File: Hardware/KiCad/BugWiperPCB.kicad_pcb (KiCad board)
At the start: 2 copper layers, 121.9 x 50.8 mm, 56 parts, among them J1 UJ20-C-H-G-SMT-1-P16-TR, Q1 NMOS_SO-8, U1 ESP32-S3-WROOM-1, U2 BTN9960LV, U3 BTN9960LV, U5 WE-TVS-82400102

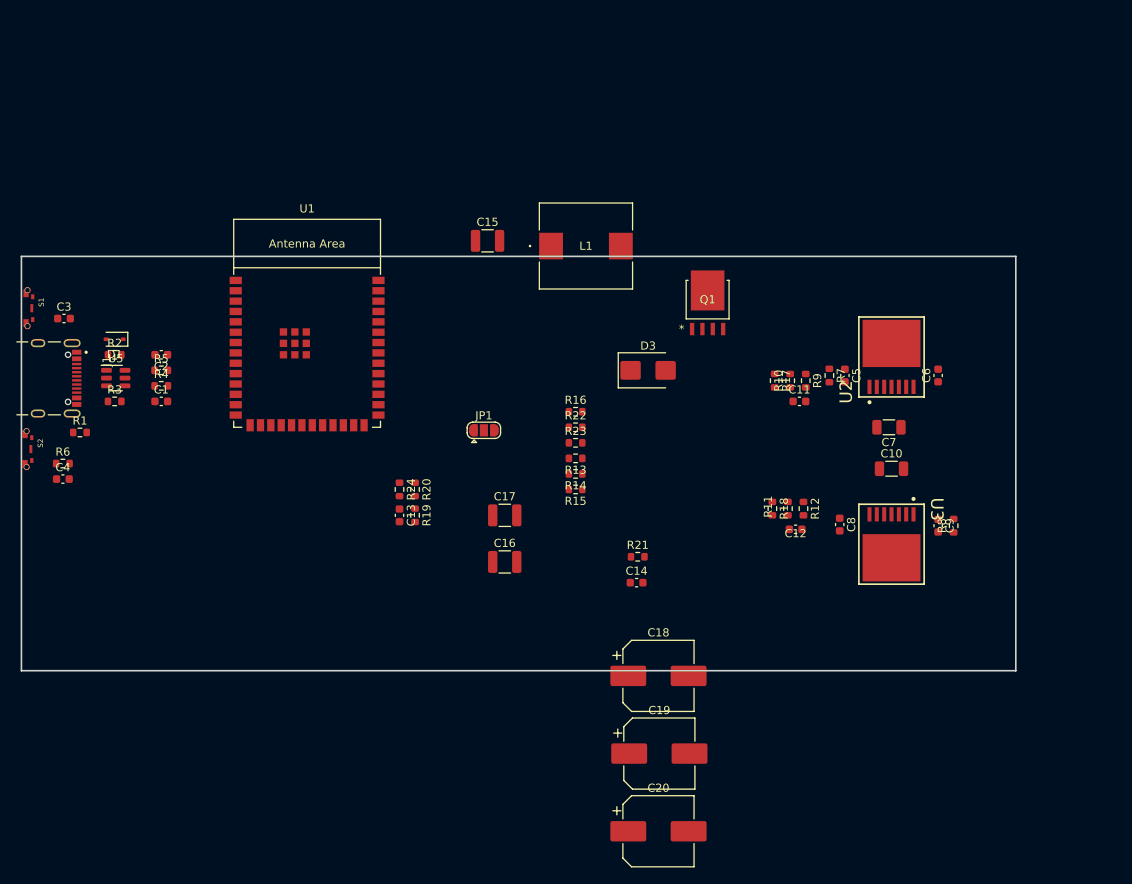
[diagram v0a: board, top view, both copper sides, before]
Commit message: Update PCB
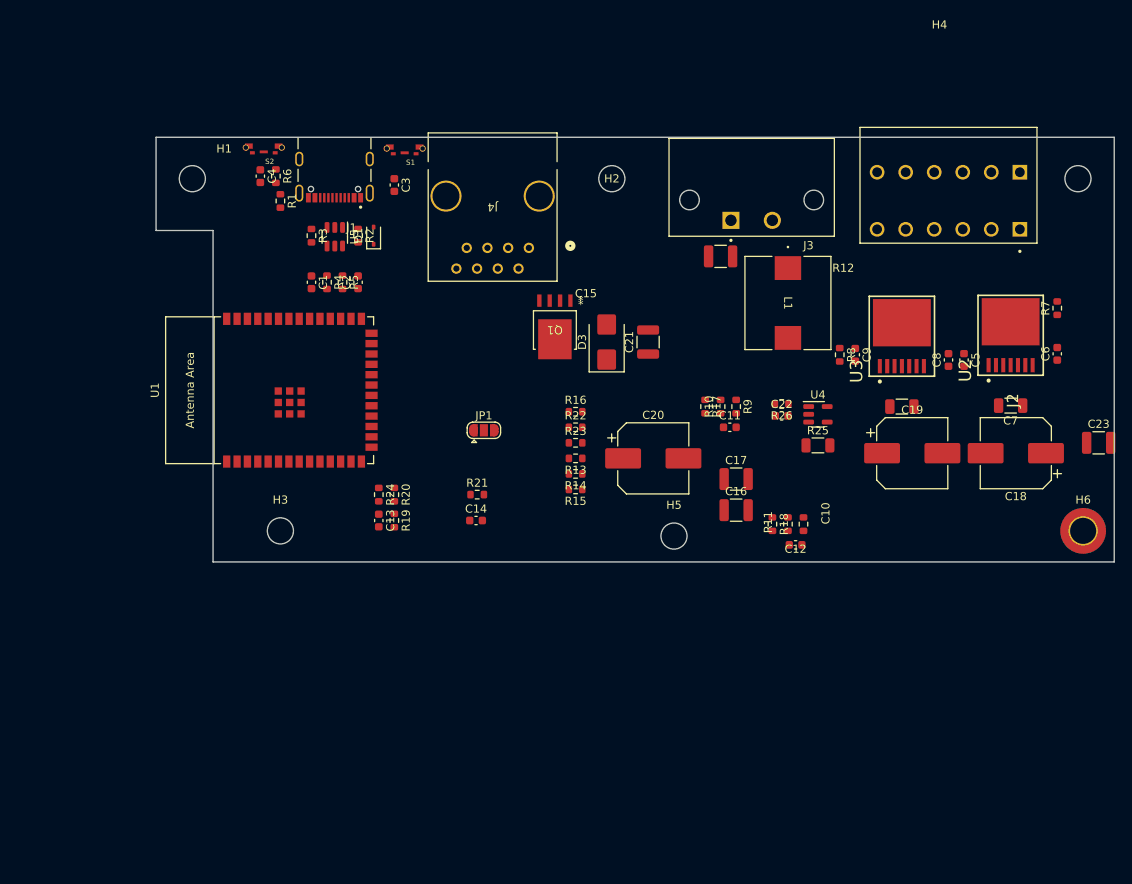
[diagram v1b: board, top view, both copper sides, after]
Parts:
- added C21: 25uF, Capacitor_SMD:C_1210_3225Metric, F.Cu at (167.0, 45.4)
- added C22: 100nF, Capacitor_SMD:C_0603_1608Metric, F.Cu at (183.4, 54.5)
- added C23: 25uF, Capacitor_SMD:C_1210_3225Metric, F.Cu at (222.2, 57.8)
- added H1: MountingHole, MountingHole:MountingHole_3.2mm_M3_DIN965, F.Cu at (111.1, 25.4)
- added H2: MountingHole, MountingHole:MountingHole_3.2mm_M3_DIN965, F.Cu at (162.6, 25.4)
- added H3: MountingHole, MountingHole:MountingHole_3.2mm_M3_DIN965, F.Cu at (121.9, 68.6)
- added H4: MountingHole, MountingHole:MountingHole_3.2mm_M3_DIN965, F.Cu at (219.7, 25.4)
- added H5: MountingHole, MountingHole:MountingHole_3.2mm_M3_DIN965, F.Cu at (170.2, 69.2)
- added H6: MountingHole_Pad, MountingHole:MountingHole_3.2mm_M3_DIN965_Pad_TopBottom, F.Cu at (220.3, 68.6)
- added J2: TBLH10-350-06BK, TBLH10_350_06BK-2:CUI_TBLH10-350-06BK, F.Cu at (212.6, 31.6)
- added J3: Phoenix_1776508, BugWiper_lib:PHOENIX_1776508, F.Cu at (189.8, 20.5)
- added J4: RJ45, BugWiper_lib:CONN8_2-908LF_AMP, F.Cu at (152.4, 33.9)
- added R25: R004, Resistor_SMD:R_1206_3216Metric, F.Cu at (187.8, 58.1)
- added R26: 1k, Resistor_SMD:R_0603_1608Metric, F.Cu at (183.4, 53.0)
- added U4: INA180A2, Package_TO_SOT_SMD:SOT-23-5, F.Cu at (187.8, 54.3)
- R21: value 1ok -> 10k
- moved C18 51.6 mm to (212.1, 59.1), turned to 180 degrees
- moved S1 51.1 mm to (137.2, 21.0), turned to 180 degrees
- moved J1 48.9 mm to (128.6, 20.4), turned to 180 degrees
- moved C19 48.1 mm to (199.4, 59.1)
- moved S2 48.0 mm to (119.9, 20.9), turned to 180 degrees
- moved C20 45.7 mm to (167.6, 59.7)
- moved C4 44.3 mm to (119.5, 25.1), turned to -90 degrees
- moved R6 43.9 mm to (121.4, 25.1), turned to -90 degrees
- moved C3 43.7 mm to (135.9, 26.2), turned to -90 degrees
- moved R1 37.5 mm to (121.9, 28.1), turned to -90 degrees
- moved D1 34.2 mm to (133.3, 32.4), turned to 90 degrees
- moved R2 33.2 mm to (131.4, 32.4), turned to -90 degrees
- moved U5 32.0 mm to (128.6, 32.5), turned to -90 degrees
- moved R3 31.5 mm to (125.7, 32.4), turned to -90 degrees
- moved R7 29.1 mm to (217.2, 41.3), turned to 90 degrees
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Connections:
- C10 pad 1: +12V -> +12V_HighSide
- C19 pad 1: +12V -> +12V_HighSide
- C20 pad 1: +12V -> +12V_HighSide
- C6 pad 1: +12V -> +12V_HighSide
- C7 pad 1: +12V -> +12V_HighSide
- C8 pad 1: +12V -> +12V_HighSide
- U2 pad 6: +12V -> +12V_HighSide
- U2 pad 7: +12V -> +12V_HighSide
- U3 pad 6: +12V -> +12V_HighSide
- U3 pad 7: +12V -> +12V_HighSide
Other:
- board size 121.9 x 50.8 mm -> 117.5 x 52.1 mm
